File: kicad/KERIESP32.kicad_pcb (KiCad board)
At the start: 2 copper layers, 76.2 x 25.4 mm, 18 parts, among them J1 USB_OTG, P1 CONN, SW1 RESET, SW2 IO0, U1 ESP-WROOM-32, U2 NJM2884, U3 FT231XS

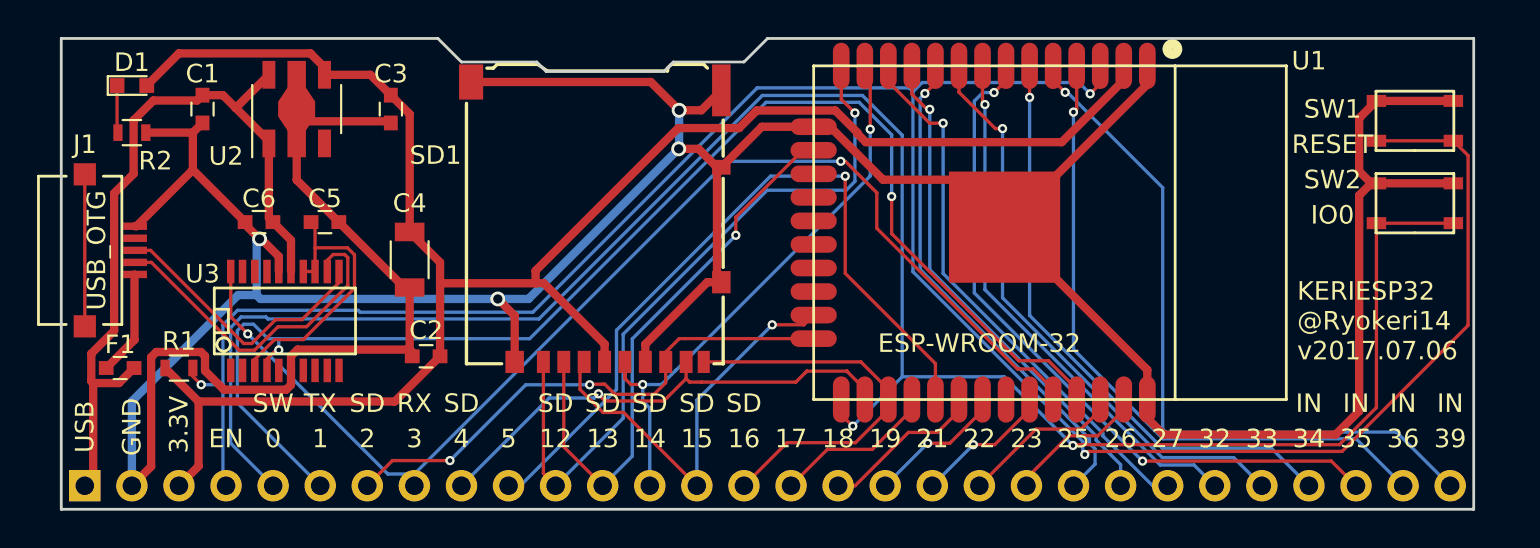
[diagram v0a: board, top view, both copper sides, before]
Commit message: 小型化，自動配線成功
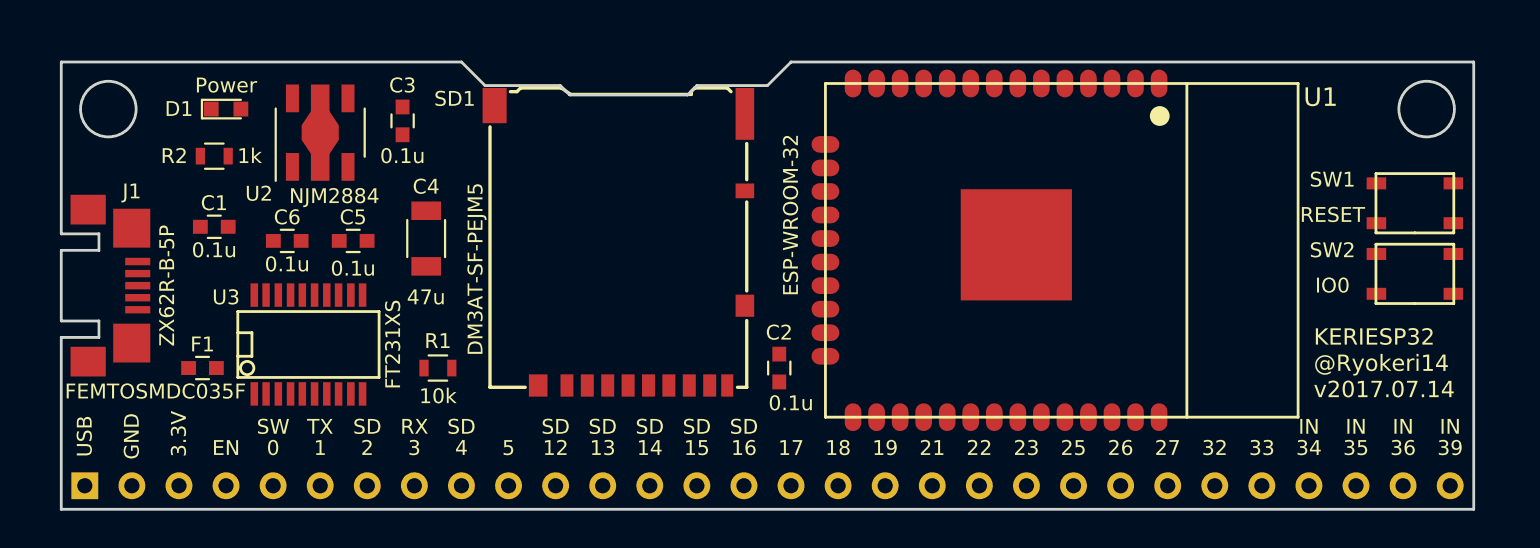
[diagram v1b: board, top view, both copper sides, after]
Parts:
- F1: value FEMTOSMDC035F-02 -> FEMTOSMDC035F
- J1: value USB_OTG -> ZX62R-B-5P
- P1: footprint Pin_Headers:Pin_Header_Straight_1x30_Pitch2.54mm -> KERIESP32:Pin_Header_Straight_1x30_Pitch2.54mm
- SD1: value Micro_SD -> DM3AT-SF-PEJM5
- moved C2 19.1 mm to (158.1, 113.0), turned to 90 degrees
- moved R1 14.0 mm to (139.7, 113.0)
- moved C1 6.38 mm to (127.6, 105.4), turned to 180 degrees
- moved D1 5.24 mm to (128.3, 99.1)
- moved R2 4.62 mm to (127.6, 101.6)
- moved SW1 4.45 mm to (192.4, 104.1)
- moved F1 4.44 mm to (127.0, 113.0)
- moved SW2 3.81 mm to (192.4, 108.0)
- moved J1 2.29 mm to (119.4, 108.6)
- moved C6 1.83 mm to (131.6, 106.2)
- moved C5 1.83 mm to (135.1, 106.2)
- moved U3 1.80 mm to (132.7, 111.8)
- moved SD1 1.80 mm to (149.9, 96.5)
- moved U2 1.80 mm to (133.3, 100.3)
- moved C4 1.45 mm to (139.1, 106.0)
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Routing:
- net GND: track 227.4 -> 0.00 mm, vias 4 -> 0
- net ENABLE: track 126.9 -> 0.00 mm, vias 3 -> 0
- net IO0: track 112.4 -> 0.00 mm, vias 2 -> 0
- net +3V3: track 102.4 -> 0.00 mm
- net TXD: track 73.4 -> 0.00 mm, vias 2 -> 0
- net RXD: track 64.7 -> 0.00 mm, vias 2 -> 0
- net +5V: track 42.4 -> 0.00 mm
- net Net-(P1-Pad10): track 41.0 -> 0.00 mm, vias 1 -> 0
- net SD_SD2: track 39.1 -> 0.00 mm, vias 1 -> 0
- net Net-(P1-Pad30): track 38.9 -> 0.00 mm, vias 1 -> 0
- net Net-(P1-Pad28): track 38.2 -> 0.00 mm, vias 2 -> 0
- net Net-(P1-Pad29): track 36.2 -> 0.00 mm, vias 1 -> 0
- net Net-(P1-Pad27): track 32.3 -> 0.00 mm, vias 1 -> 0
- net Net-(P1-Pad26): track 31.9 -> 0.00 mm, vias 1 -> 0
- net SD_CLK: track 31.7 -> 0.00 mm, vias 2 -> 0
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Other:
- board size 76.2 x 25.4 mm -> 76.2 x 24.1 mm
- net class Default: clearance 0.18 -> 0.16; via_dia 0.5 -> 0.6
- net class Power: clearance 0.18 -> 0.16
- rule trace_clearance: 0.18 -> 0.16
- rule trace_min: 0.18 -> 0.16
- rule via_min_size: 0.4 -> 0.6
- board text added: "KERIESP32 @Ryokeri14 v2017.07.14"
- board text removed: "KERIESP32 @Ryokeri14 v2017.07.06"
